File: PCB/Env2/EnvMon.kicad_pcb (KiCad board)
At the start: 2 copper layers, 70 x 70 mm, 51 parts, among them J1 LCD, J10 Conn_01x01, J11 Conn_01x01, J12 Conn_01x01, J2 DC, J3 TEMP, J4 LCD, J5 Reset, J6 USB-C-Socket-H, J7 TC2030-USB-NL-DS, J8 T6793, J9 Conn_01x01, U1 ESP32-S3-MINI-1, U2 SCD41, U3 MD8942, U4 MCP9808_MSOP, U5 GZP6816D, U8 VEML6040

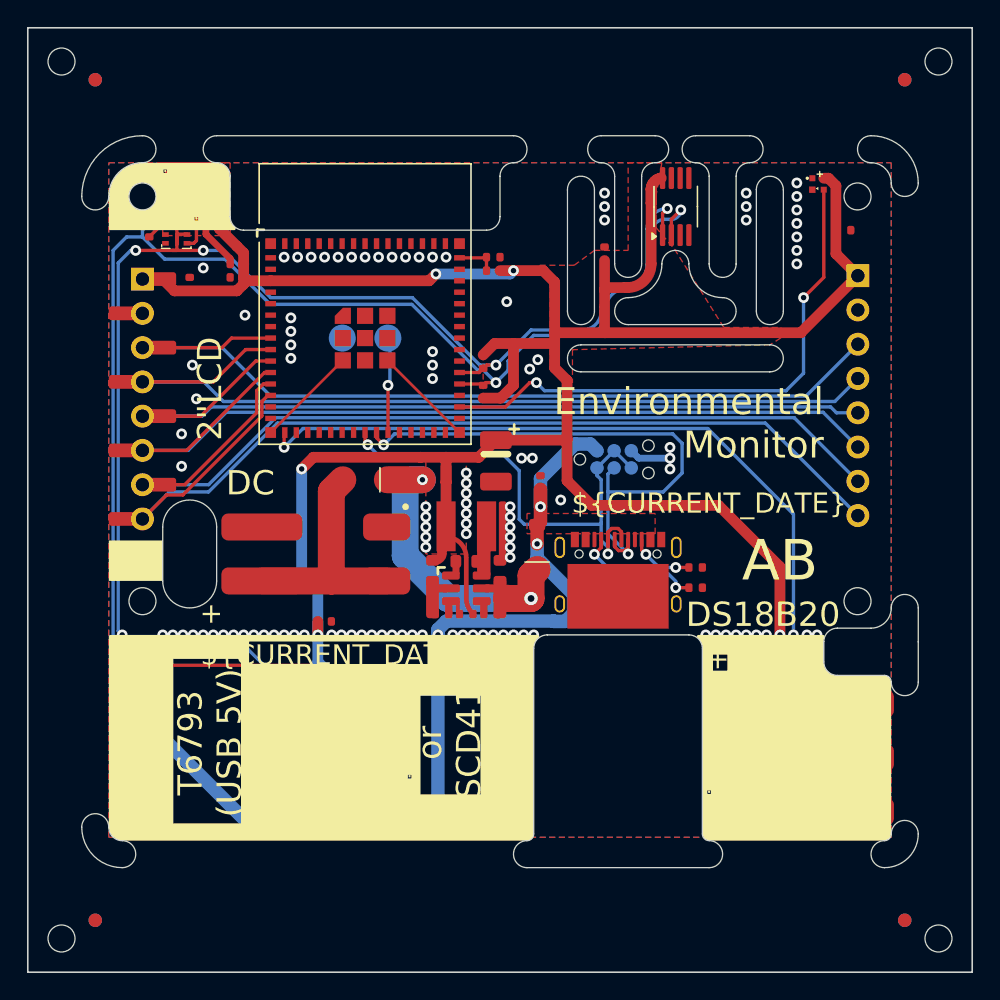
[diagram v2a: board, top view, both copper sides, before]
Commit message: Library update
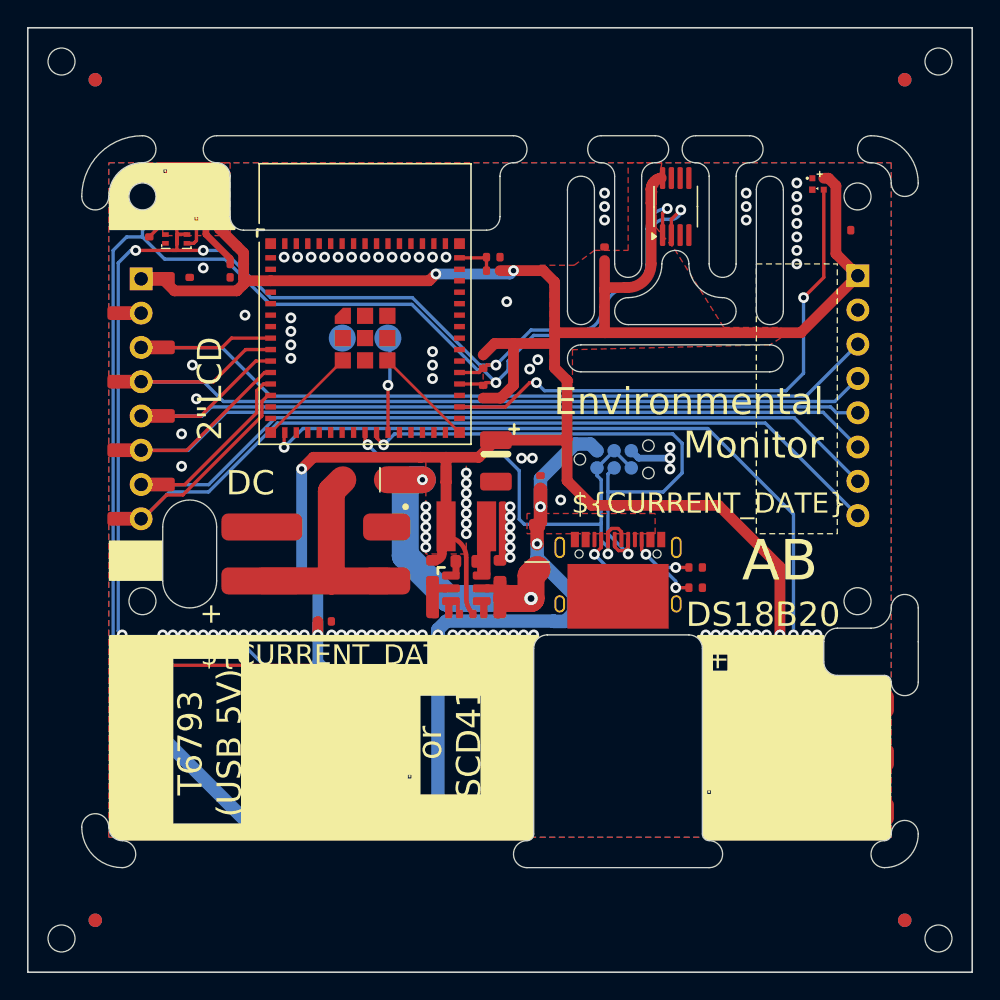
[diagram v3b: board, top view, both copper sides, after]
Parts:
- J1: footprint RevK:PinSocket_1x08_P2.54mm_Vertical_SMD -> RevK:LCD2
- moved J1 0.10 mm to (73.4, 83.6)
